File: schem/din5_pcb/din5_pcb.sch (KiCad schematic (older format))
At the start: 10 parts, among them J101 2x3 female, J102 2x3 female, U101 74HCT245, U102 74HC165, U103 74HC595, U104 74HC595

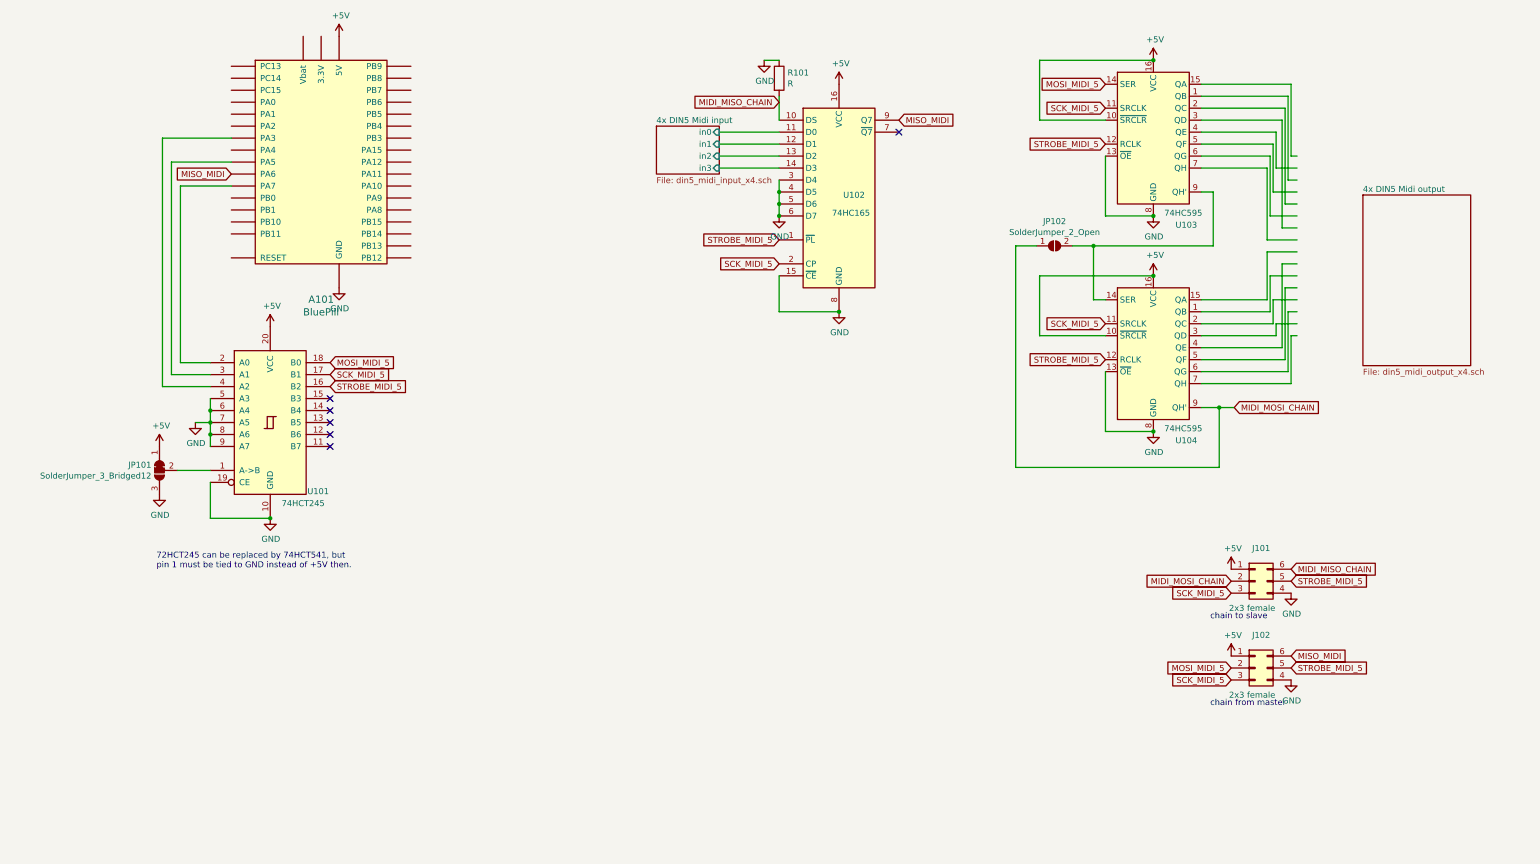
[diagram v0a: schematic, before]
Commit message: din5 pcb ++
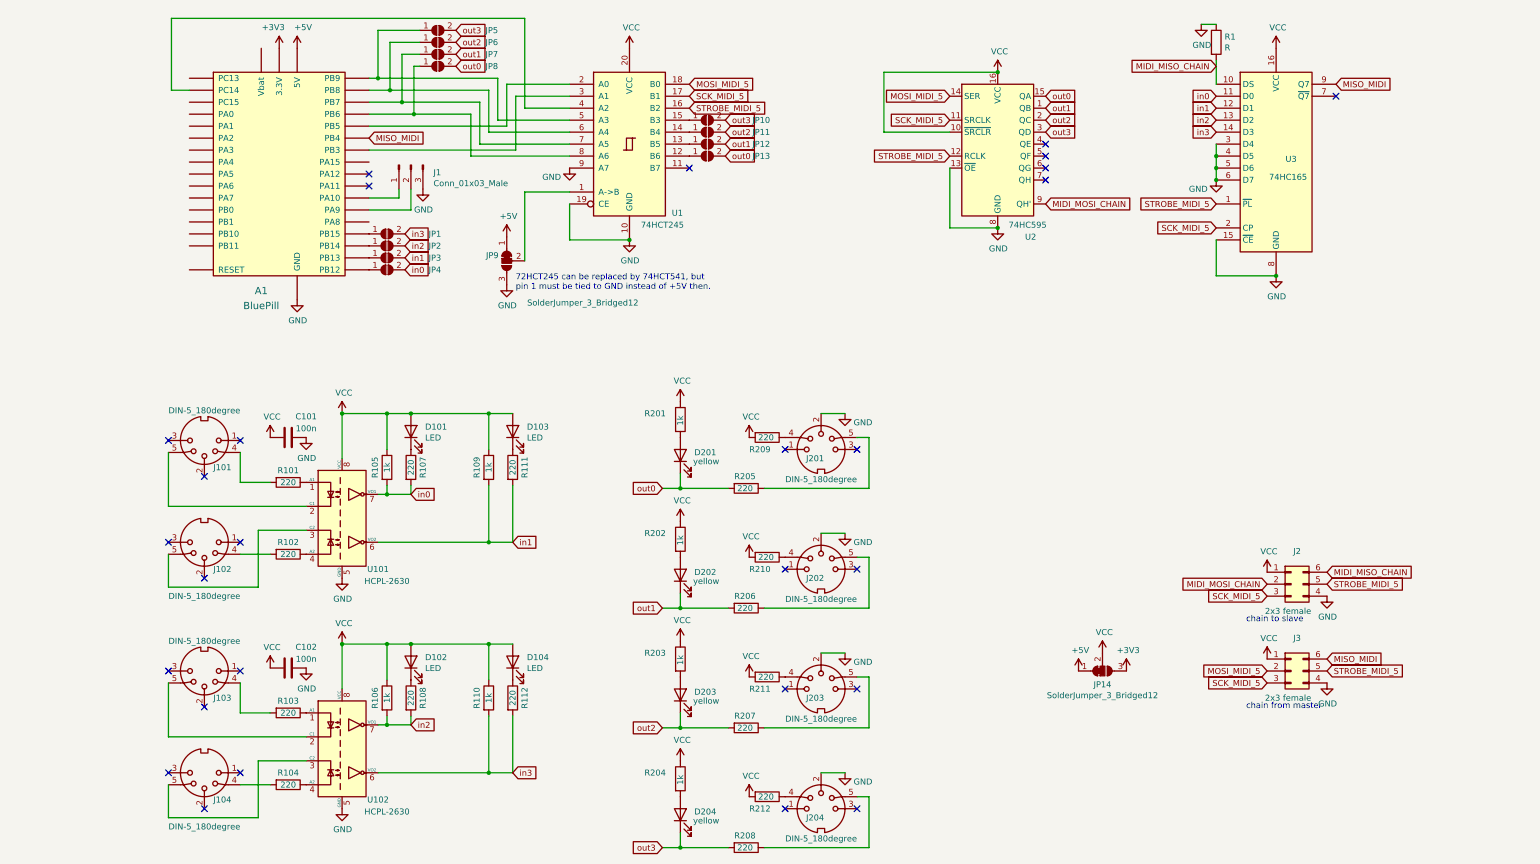
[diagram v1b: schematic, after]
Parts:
- removed JP102: SolderJumper_2_Open, Jumper:SolderJumper-2_P1.3mm_Open_TrianglePad1.0x1.5mm, symbol Jumper:SolderJumper_2_Open
- removed U104: 74HC595, Package_DIP:DIP-16_W7.62mm, symbol 74xx:74HC595
- added C101, C102: 100n, Capacitor_SMD:C_0805_2012Metric, symbol Device:C
- added D101, D102, D103: LED, LED_THT:LED_D3.0mm_Horizontal_O1.27mm_Z2.0mm, symbol Device:LED
- added D104: LED, LED_THT:LED_D3.0mm_Horizontal_O3.81mm_Z6.0mm, symbol Device:LED
- added D201, D202, D203, D204: yellow, LED_THT:LED_D3.0mm_Horizontal_O3.81mm_Z6.0mm, symbol Device:LED
- added J1: Conn_01x03_Male, Connector_PinHeader_2.54mm:PinHeader_1x03_P2.54mm_Vertical, symbol Connector:Conn_01x03_Male
- added J101, J102, J103, J104, J201, J202, J203, J204: DIN-5_180degree, footprints:DIN5, symbol Connector:DIN-5_180degree
- added JP1, JP10, JP11, JP12, JP13, JP2, JP3, JP4, JP5, JP6, JP7, JP8: SolderJumper_2_Open, Jumper:SolderJumper-2_P1.3mm_Open_TrianglePad1.0x1.5mm, symbol Jumper:SolderJumper_2_Open
- added JP14: SolderJumper_3_Bridged12, Jumper:SolderJumper-3_P1.3mm_Bridged12_RoundedPad1.0x1.5mm, symbol Jumper:SolderJumper_3_Bridged12
- added R101, R102, R103, R104, R107, R108, R111, R112, R205, R206, R207, R208, R209, R210, R211, R212: 220, Resistor_SMD:R_0805_2012Metric, symbol Device:R
- added R105, R106, R109, R110, R201, R202, R203, R204: 1k, Resistor_SMD:R_0805_2012Metric, symbol Device:R
- added U101, U102: HCPL-2630, Package_DIP:DIP-8_W7.62mm, symbol Isolator:HCPL-2630
- JP9: renamed from JP101; footprint Jumper:SolderJumper-3_P2.0mm_Open_TrianglePad1.0x1.5mm -> Jumper:SolderJumper-3_P1.3mm_Bridged12_RoundedPad1.0x1.5mm
- renumbered A101 to A1, J101 to J2, J102 to J3, R101 to R1, U101 to U1, U103 to U2, U102 to U3
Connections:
- net labels added: +3V3, VCC, in0, in1, in2, in3, out0, out1, out2, out3
- wire segments 98 -> 131
- no-connect marks 6 -> 28
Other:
- moved on the sheet: A1, J2, J3, JP9, R1, U1, U2, U3
